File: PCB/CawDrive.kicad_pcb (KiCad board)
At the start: 4 copper layers, 50 x 42 mm, 109 parts, among them CN2 WAFER-SH1.0-6PWB, CN3 WAFER-SH1.0-4PWB, Q10 TPH3R704PL, Q11 TPH3R704PL, Q12 TPH3R704PL, Q7 TPH3R704PL, Q8 TPH3R704PL, Q9 TPH3R704PL, U1 TJA1051T/3/1J, U10 WAFER-SH1.0-2PWB, U11 WAFER-SH1.0-2PWB, U12 WAFER-SH1.0-2PWB, U2 TLV76733DRVR, U5 WAFER-SH1.0-2PWB, U6 WAFER-SH1.0-2PWB, U7 DRV8323RSRGZR, U8 STM32F446RETx, U9 MT6835GT-STD, X1 CSTNE16M0V530000R0

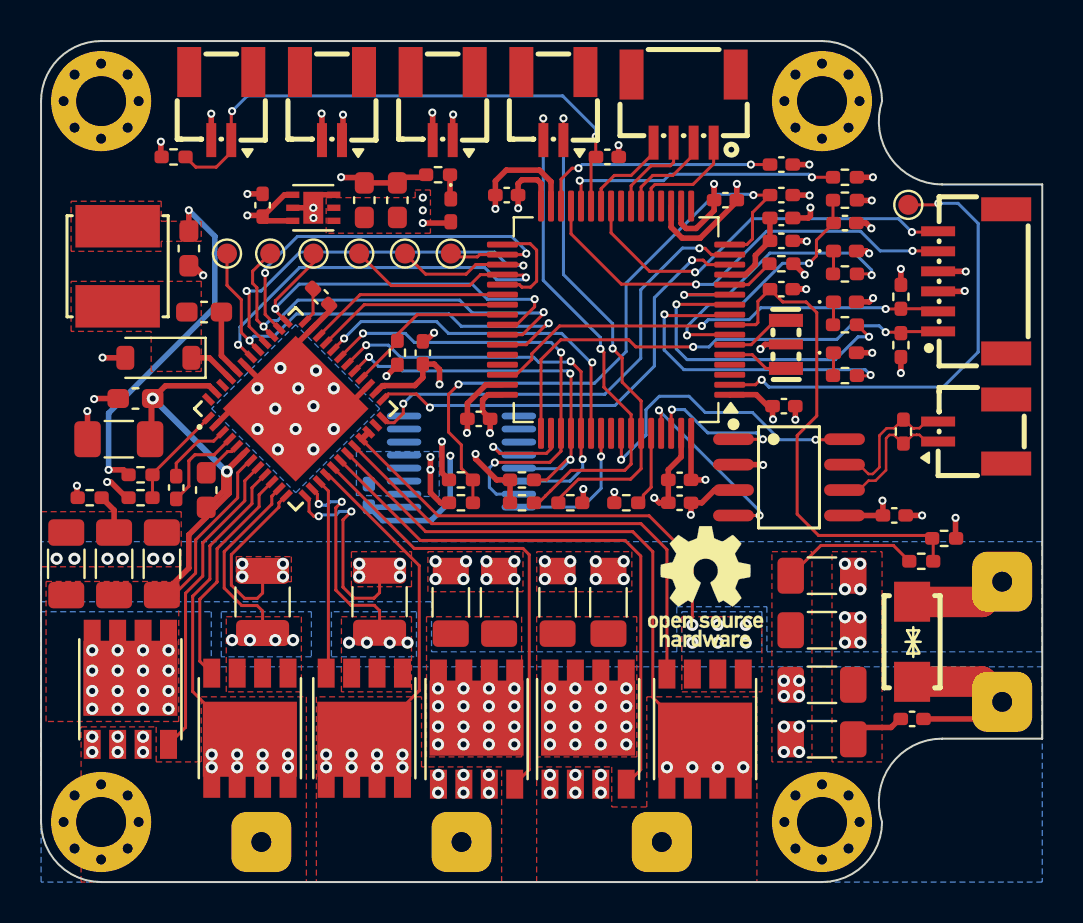
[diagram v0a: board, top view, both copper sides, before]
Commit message: 优化PCB
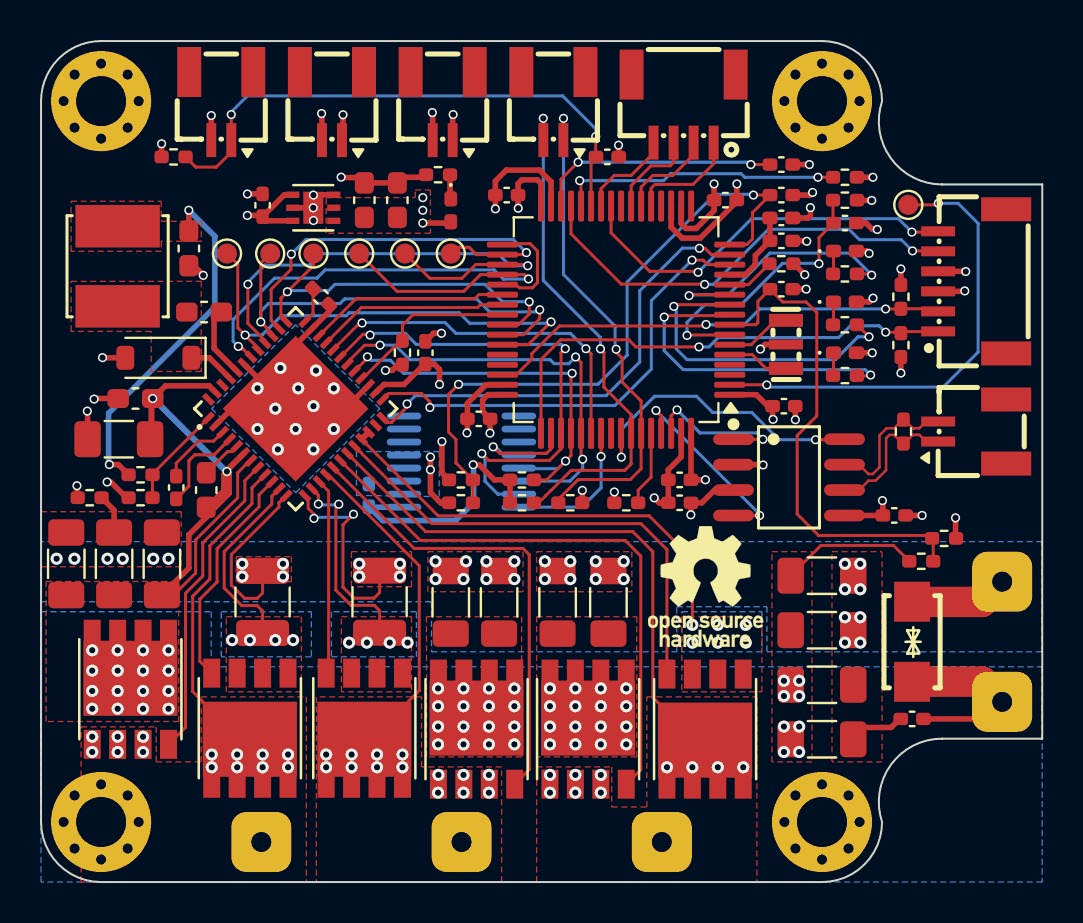
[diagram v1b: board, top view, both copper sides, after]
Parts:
- moved R17 0.25 mm to (138.0, 83.6)
- moved C32 0.13 mm to (139.2, 83.6)
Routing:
- net /TIM1_CH1: track 20.6 -> 18.9 mm
- net /SPI3_SCK: track 23.4 -> 24.9 mm
- net /TIM1_CH3N: track 26.9 -> 27.9 mm
- net /TIM1_CH2N: track 24.4 -> 25.2 mm
- net GND: track 68.5 -> 69.1 mm, vias 48 -> 49
- net /TIM1_CH1N: track 21.3 -> 20.7 mm
- net /MCU_STA: track 13.9 -> 13.3 mm
- net /SPI3_MOSI: track 21.0 -> 21.5 mm
- net +3.3V: track 52.7 -> 52.8 mm, vias 24 -> 23
